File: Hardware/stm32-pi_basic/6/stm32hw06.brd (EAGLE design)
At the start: 149.4 x 77.7 mm, 53 parts

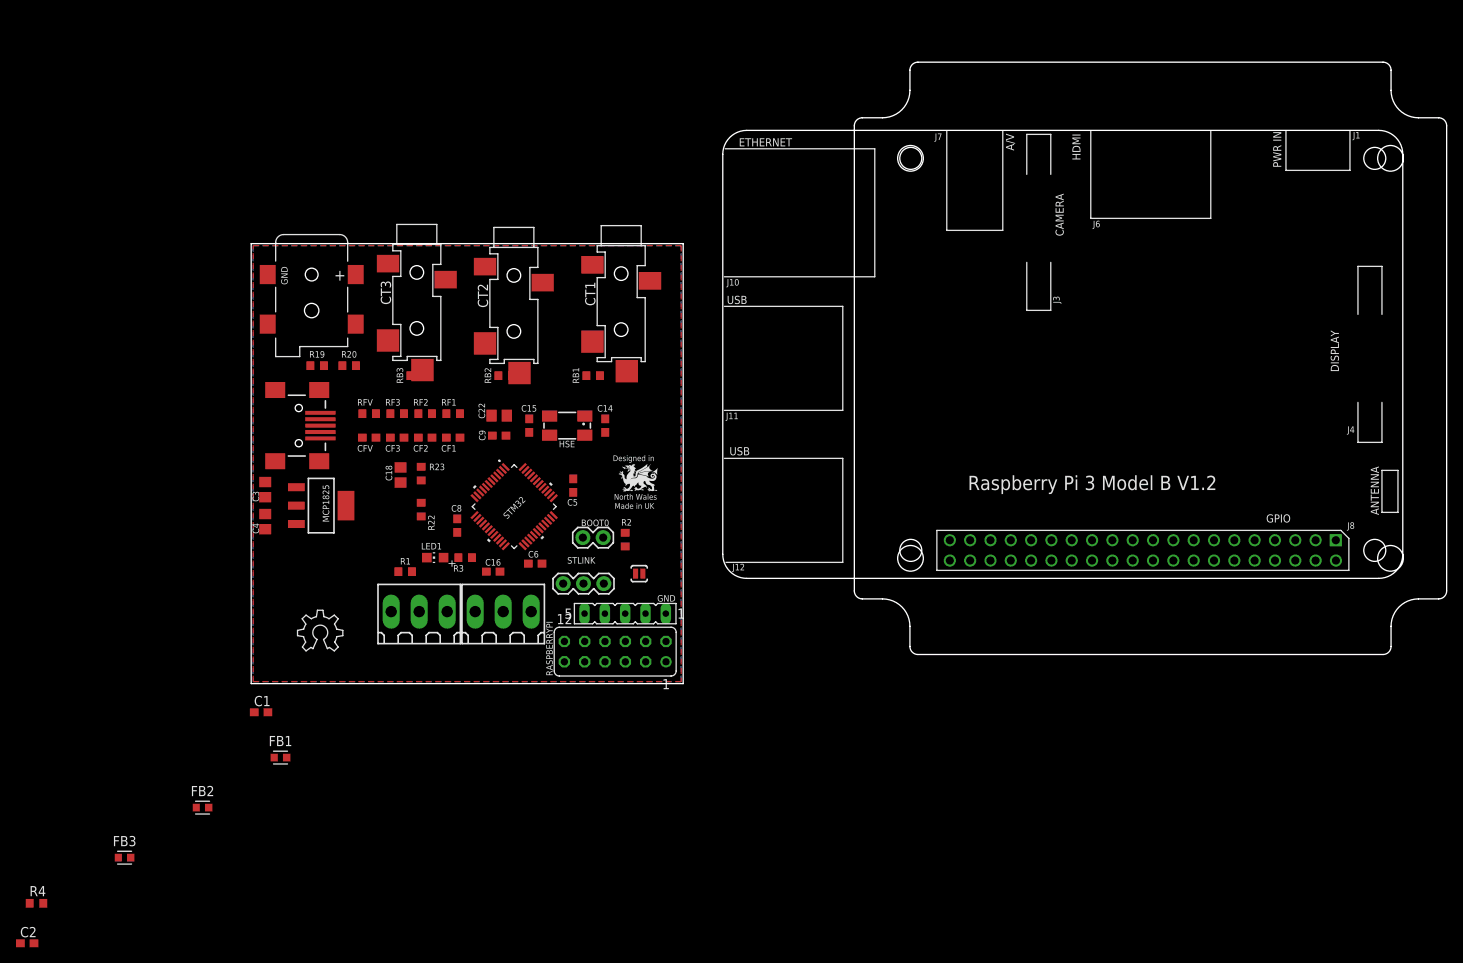
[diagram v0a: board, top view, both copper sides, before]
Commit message: sync
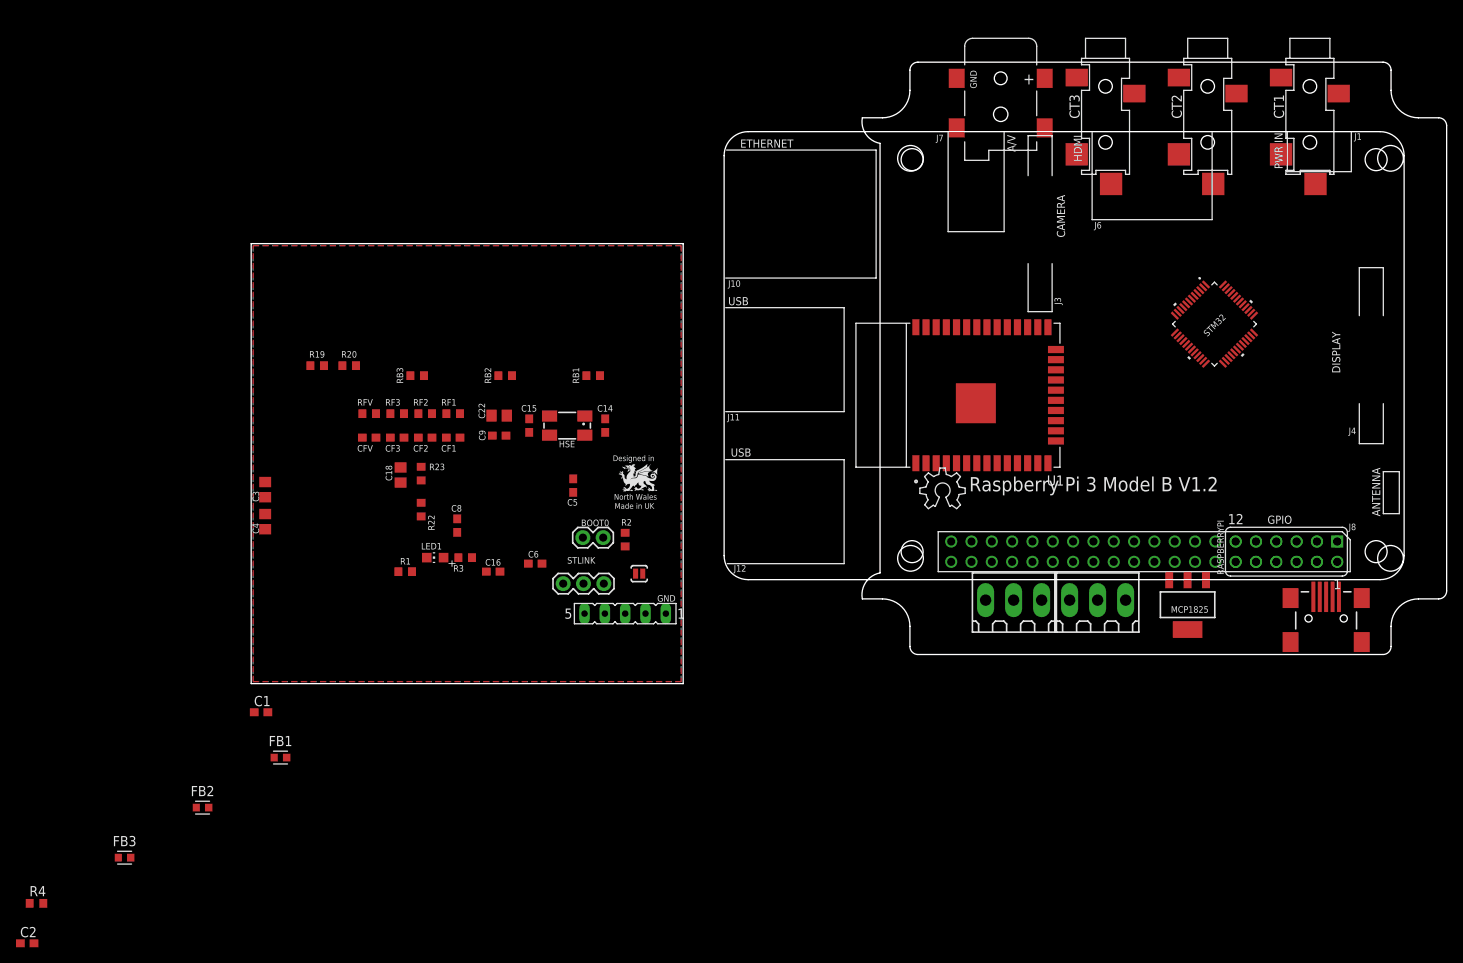
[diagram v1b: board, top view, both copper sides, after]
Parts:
- added U1: ESP32-WROOM-32D, ESP32-WROOM-32D:MODULE_ESP32-WROOM-32D
- moved U$10 136.8 mm to (134.4, 2.95), turned to 90 degrees
- moved MCP1825 109.0 mm to (117.0, 9.86), turned to 180 degrees
- moved STM32 90.5 mm to (120.4, 44.9)
- moved CT2 89.9 mm to (119.6, 78.2)
- moved U$1 89.6 mm to (93.7, 75.7)
- moved CT1 89.2 mm to (132.3, 78.2)
- moved CT3 89.2 mm to (106.8, 78.2)
- moved RASPBERRYPI 84.8 mm to (129.4, 16.5)
- moved LOGO1 79.8 mm to (83.6, 21.9)
- moved DS18B20 74.3 mm to (95.3, 10.4)
- moved PULSE 74.3 mm to (105.8, 10.4)
- moved PCB1 0.23 mm to (144.1, 69.0)
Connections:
- new net 3V3: U1.2
- net GND: now also U1.1, U1.15, U1.38, U1.39
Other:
- outline, holes or cut-outs redrawn
- board text added: "emonSTM32mini"
- board text added: "v0.2"
- board text removed: "emonSTM32"
- board text removed: "v0.1"

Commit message: sync
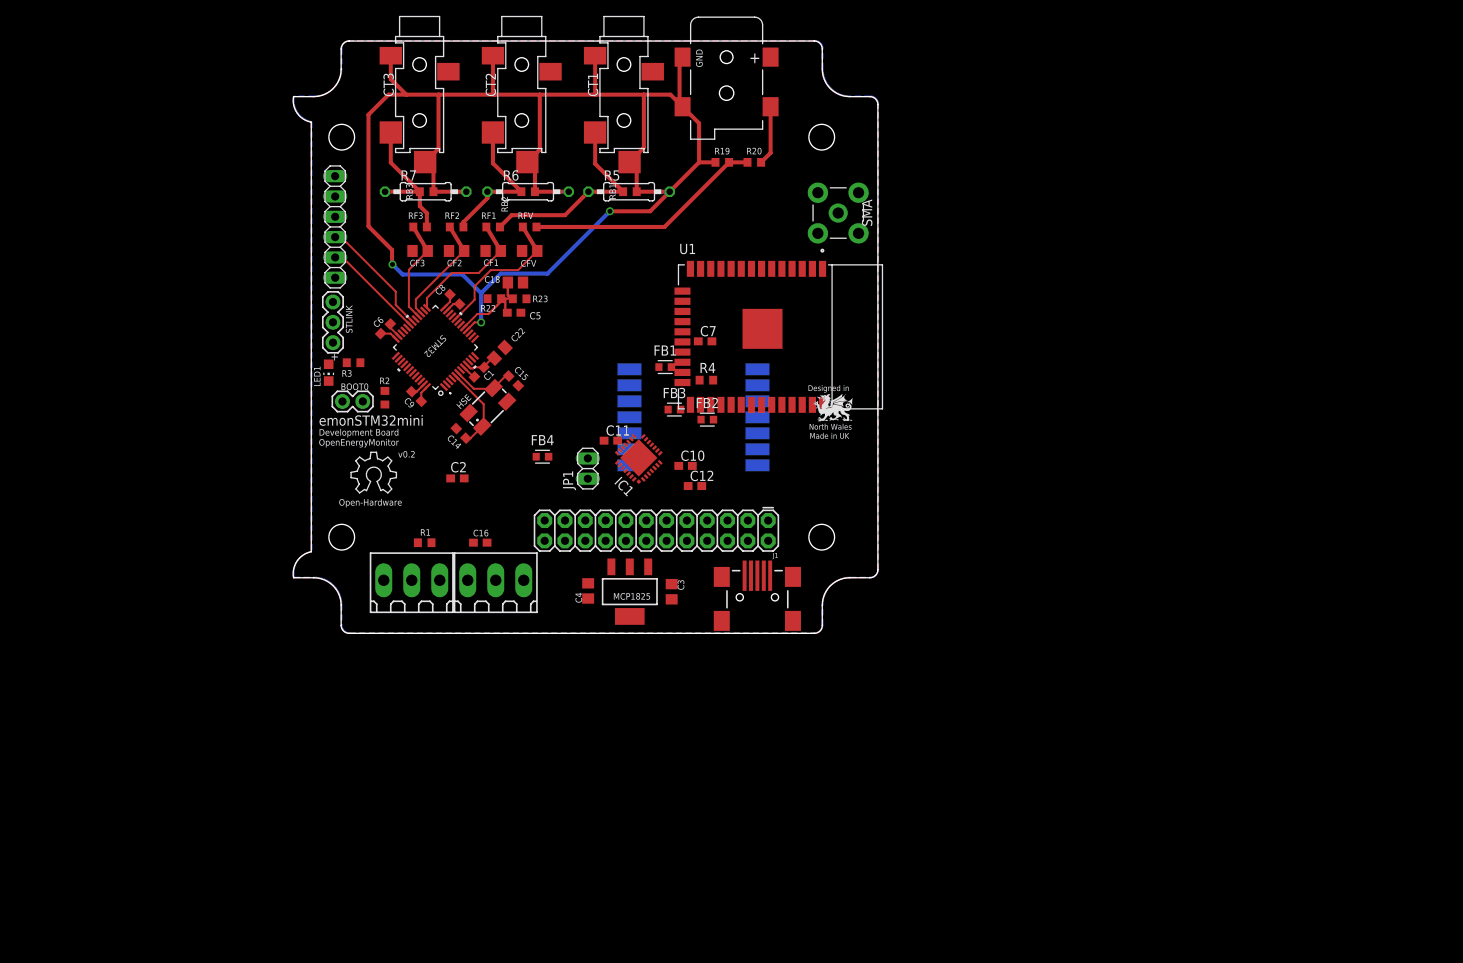
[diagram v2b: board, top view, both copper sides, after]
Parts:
- removed GND: UART, con-lsta:FE05-1
- removed PCB1: RPI3RPI3, e14_Rpi3_RevA+mirror-pcb:RPI3
- removed RASPBERRYPI: (no value), con-lsta:FE06-2
- removed SJ1: SOLDERJUMPERNO, SparkFun:SJ_2S-NO
- added C10, C11, C7: 100nF, rcl:C0603
- added C12: 2.2uF, rcl:C0603
- added FB4: FBCHIP-0603(1608-METRIC), Filter:BEADC1608X95N
- added IC1: CP2102, silabs:MLP28
- added J1: CONN_12X2, SparkFun-Connectors:2X12
- added JP1: PINHD-1X2, Connector:1X02
- added JP2: UART_STM, Connector:1X06
- added R5, R6, R7: (no value), rcl:0207/10
- added SMA: 5-1814400-1, 5-1814400-1 sma connector:518144001
- added U$2: RFM12_SMDSMD, rfm12b _ rfm69cw:RFM12
- CF1, CF2, CF3, CFV: value 100nF -> 10nF; device resistor:C0603 -> rcl:C0805
- RB2, RB3: value 22r -> 6R8
- RF1, RF2, RF3, RFV: value 330R -> 9k1
- moved R4 106.3 mm to (56.9, 37.9)
- moved STM32 97.4 mm to (23.0, 42.0), turned to 135 degrees
- moved FB3 88.7 mm to (52.9, 34.3)
- moved CT3 85.8 mm to (21.0, 80.9)
- moved CT1 85.8 mm to (46.6, 80.9)
- moved CT2 85.8 mm to (33.8, 80.9)
- moved FB2 79.6 mm to (57.0, 33.0)
- moved C2 79.2 mm to (25.8, 25.7)
- moved DS18B20 75.3 mm to (20.1, 12.9)
- moved PULSE 75.3 mm to (30.6, 12.9)
- moved U$10 71.1 mm to (63.3, 5.59)
- moved LOGO1 71.1 mm to (12.5, 23.8)
- moved MCP1825 69.7 mm to (47.3, 11.5)
- moved FB1 68.5 mm to (51.8, 39.6)
- moved R19 56.7 mm to (58.9, 65.2)
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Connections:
- removed net 3V3: U1.2
- new net +3V3RPI: J1.1, J1.17
- new net AGND: C1.2, C22.2, FB4.1, STM32.8
- new net CLK_RPI: J1.23
- new net CS_RPI: J1.24
- new net D+: IC1.4, U$10.D+
- new net D-: IC1.5, U$10.D-
- new net ESP_BOOT0: U1.25
- new net ESP_RST: U1.3
- new net ESP_RX: U1.34
- new net ESP_TX: U1.35
- new net MISO_RPI: J1.21
- new net MOSI_RPI: J1.19
- new net N$11: U$2.14
- new net N$13: U$2.2
- new net N$14: U$2.12
- new net N$15: U$2.1
- new net N$16: U$2.13
- new net N$17: U$2.6
- new net N$18: SMA.1, U$2.8
- new net N$19: JP2.5
- new net N$5: J1.9
- new net SCL: J1.5, STM32.45, U1.36
- new net SDA: J1.3, STM32.46, U1.33
- new net SPI3_CLK: STM32.39
- new net SPI3_MISO: STM32.40
- new net SPI3_MOSI: STM32.41
- new net SPI3_NSS: STM32.38
- new net STM_RX: J1.8, JP2.2, STM32.31
- new net STM_TX: J1.10, JP2.3, STM32.30
- net +3V3: now also C11.1, IC1.6, U$2.9, U1.2; no longer C5.1, SJ1.2, STM32.9
- net +3V3ANA: now also STM32.9
- net +5V: now also C10.1, C12.1, IC1.7, IC1.8, J1.2, J1.4, JP2.4; no longer GND.3, RASPBERRYPI.1, RASPBERRYPI.3
- net BIAS: now also R5.2, R6.2, R7.2
- net BIAS_IN: now also C5.1
- net BOOT0: now also IC1.28, J1.7; no longer RASPBERRYPI.8
- net CT1: now also STM32.25; no longer STM32.10
- net CT2: now also CF2.1, STM32.27; no longer CF2.2, STM32.11
- net CT3: now also CF3.1, STM32.28; no longer CF3.2, STM32.12
- net GND: now also C10.2, C11.2, C12.2, C7.2, CF2.2, CF3.2, FB4.2, IC1.3, IC1.EXP, IC1.M, J1.14, J1.20, J1.6, JP2.6, SMA.2, SMA.3, SMA.4, SMA.5, U$2.10, U$2.7; no longer C1.2, C22.2, CF2.1, CF3.1, GND.1, RASPBERRYPI.10, RASPBERRYPI.5, STM32.8
- net LED: now also STM32.42; no longer STM32.27
- net N$1: now also IC1.9; no longer GND.2, SJ1.1
- net N$10: now also R7.1
- net N$2: now also R5.1
- net N$8: now also R6.1
- net PULSE: now also C7.1, STM32.43; no longer STM32.28
- net RST_STM: now also IC1.24, J1.11, JP2.1; no longer RASPBERRYPI.12
- net UART_RX: now also IC1.26, JP1.1; no longer GND.4, RASPBERRYPI.7, STM32.31
- net UART_TX: now also IC1.25, JP1.2; no longer GND.5, RASPBERRYPI.9, STM32.30
- net VSIG: now also STM32.20; no longer STM32.25
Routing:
- net BIAS: track 0.00 -> 197.3 mm, vias 0 -> 3
- net ADC0: track 0.00 -> 29.7 mm
- net N$2: track 0.00 -> 26.1 mm
- net N$8: track 0.00 -> 18.8 mm
- net VSIG: track 0.00 -> 18.3 mm
- net N$10: track 0.00 -> 18.0 mm
- net CT1: track 0.00 -> 16.4 mm
- net STM_TX: track 0.00 -> 15.1 mm
- net CT2: track 0.00 -> 14.1 mm
- net CT3: track 0.00 -> 13.1 mm
- net STM_RX: track 0.00 -> 12.8 mm
- net BIAS_IN: track 0.00 -> 11.9 mm
- net HSE_IN: track 0.00 -> 10.5 mm
- net HSE_OUT: track 0.00 -> 7.82 mm
- net AC: track 0.00 -> 7.44 mm
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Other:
- board size 149.4 x 77.7 mm -> 73.1 x 74 mm
- board text added: "Rx"
- board text added: "Tx"
- board text removed: "3.3"
- board text removed: "RX"
- board text removed: "TX"
